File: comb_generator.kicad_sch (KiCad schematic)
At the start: 61 parts, among them J11 RFShield_TwoPieces, J2 RFShield_TwoPieces, U1 ISL3280ExHZ, U13 PAT1220-C-3DB, U2 PHA-13HLN+, U5 Si5351C-B-GM, U6 PHA-13HLN+, U7 PAT1220-C-3DB, Y2 TG2520SMN-xx.xxxxxxMhz-xxxxNM

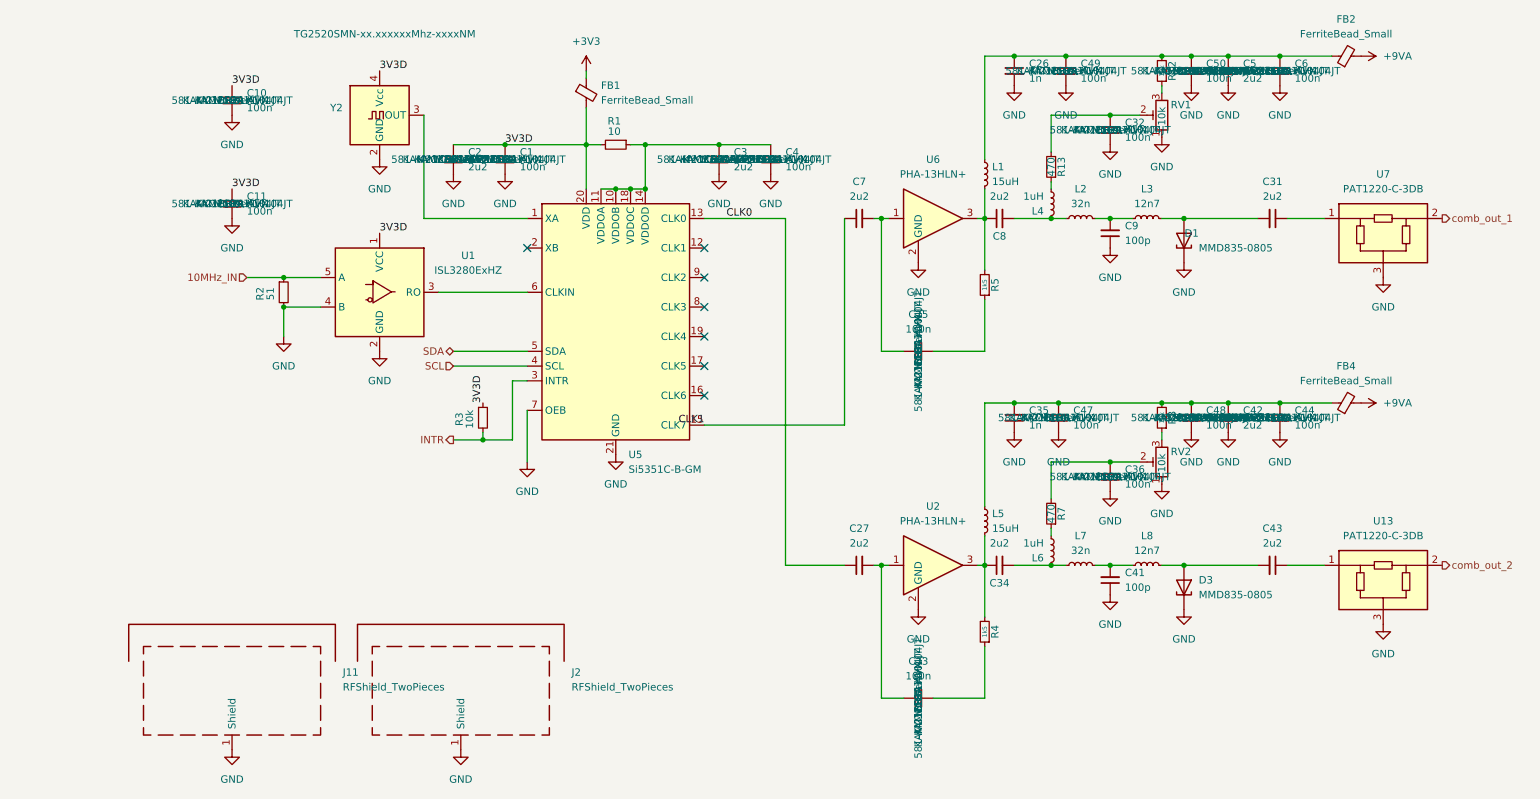
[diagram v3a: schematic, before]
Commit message: BOM...
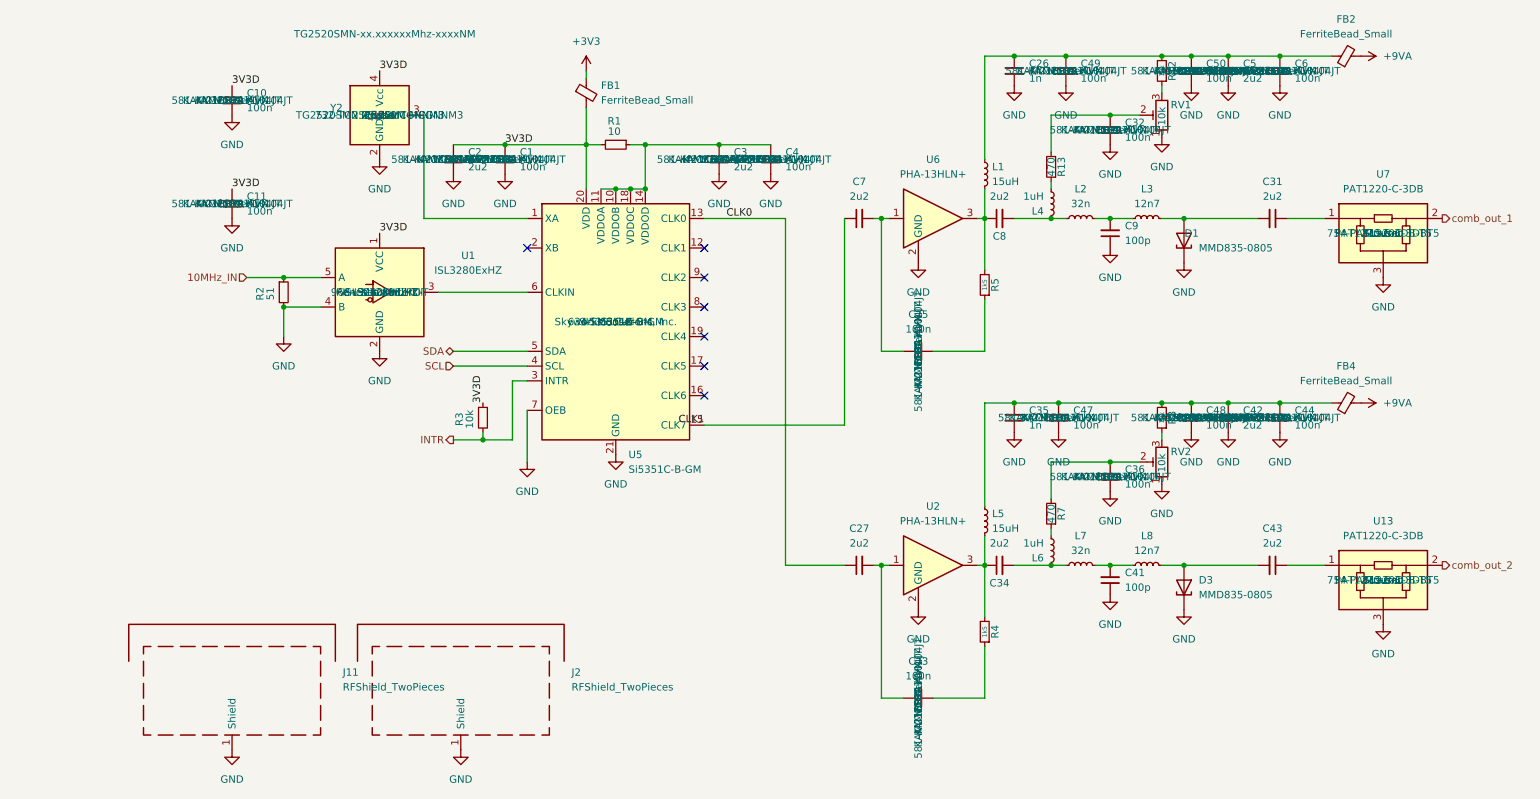
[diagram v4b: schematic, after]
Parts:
- RV1, RV2: Distributor (none) -> Mouser; Distributor PN (none) -> 652-TC33X-2-103E; Manufacturer (none) -> Bourns; Manufacturer PN (none) -> TC33X-2-103E
- U1: Distributor (none) -> Mouser; Distributor PN (none) -> 968-ISL3280EIHZ-T; Manufacturer (none) -> Renesas / Intersil; Manufacturer PN (none) -> ISL3280EIHZ-T
- U13, U7: Distributor (none) -> Mouser; Distributor PN (none) -> 754-PAT1220C-3DBT5; Manufacturer (none) -> Susumu; Manufacturer PN (none) -> PAT1220-C-3DB-T5
- U2, U6: Manufacturer (none) -> Mini-Circuits
- U5: Distributor (none) -> Mouser; Distributor PN (none) -> 634-SI5351C-B-GM; Manufacturer (none) -> Skyworks Solutions, Inc.; Manufacturer PN (none) -> SI5351C-B-GM
- Y2: Distributor (none) -> Mouser; Distributor PN (none) -> 732-TG252S25MCGNNM3; Manufacturer (none) -> Epson; Manufacturer PN (none) -> TG2520SMN 25.000M-MCGNNM3
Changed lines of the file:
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@@
 			)
 		)
+		(property "Distributor" "Mouser"
+			(at 74.93 88.9 0)
+			(effects
+				(font
+					(size 1.27 1.27)
+				)
+			)
+		)
+		(property "Distributor PN" "968-ISL3280EIHZ-T "
+			(at 74.93 88.9 0)
+			(effects
+				(font
+					(size 1.27 1.27)
+				)
+			)
+		)
+		(property "Manufacturer" "Renesas / Intersil "
+			(at 74.93 88.9 0)
+			(effects
+				(font
+					(size 1.27 1.27)
+				)
+			)
+		)
+		(property "Manufacturer PN" "ISL3280EIHZ-T "
+			(at 74.93 88.9 0)
+			(effects
+				(font
+					(size 1.27 1.27)
+				)
+			)
+		)
 		(pin "5"
 		)
@@
 			)
 		)
+		(property "Distributor" "Mouser"
+			(at 74.93 58.42 0)
+			(effects
+				(font
+					(size 1.27 1.27)
+				)
+			)
+		)
+		(property "Distributor PN" " 732-TG252S25MCGNNM3 "
+			(at 74.93 58.42 0)
+			(effects
+				(font
+					(size 1.27 1.27)
+				)
+			)
+		)
+		(property "Manufacturer" "Epson"
+			(at 74.93 58.42 0)
+			(effects
+				(font
+					(size 1.27 1.27)
+				)
+			)
+		)
+		(property "Manufacturer PN" "TG2520SMN 25.000M-MCGNNM3"
+			(at 74.93 58.42 0)
+			(effects
+				(font
+					(size 1.27 1.27)
+				)
+			)
+		)
 		(pin "2"
 		)
@@
 			)
 		)
+		(property "Distributor" "Mouser"
+			(at 115.57 93.98 0)
+			(effects
+				(font
+					(size 1.27 1.27)
+				)
+			)
+		)
+		(property "Distributor PN" " 634-SI5351C-B-GM "
+			(at 115.57 93.98 0)
+			(effects
+				(font
+					(size 1.27 1.27)
+				)
+			)
+		)
+		(property "Manufacturer" "Skyworks Solutions, Inc. "
+			(at 115.57 93.98 0)
+			(effects
+				(font
+					(size 1.27 1.27)
+				)
+			)
+		)
+		(property "Manufacturer PN" "SI5351C-B-GM"
+			(at 115.57 93.98 0)
+			(effects
+				(font
+					(size 1.27 1.27)
+				)
+			)
+		)
 		(pin "9"
 		)
@@
 			)
 		)
-		(property "Manufacturer PN" ""
+		(property "Manufacturer PN" "TC33X-2-103E"
 			(at 209.55 118.11 0)
 			(effects
@@
 			)
 		)
-		(property "Manufacturer" ""
+		(property "Manufacturer" "Bourns "
 			(at 209.55 118.11 0)
 			(effects
@@
 			)
 		)
-		(property "Distributor" ""
+		(property "Distributor" "Mouser"
 			(at 209.55 118.11 0)
 			(effects
@@
 			)
 		)
-		(property "Distributor PN" ""
+		(property "Distributor PN" " 652-TC33X-2-103E "
 			(at 209.55 118.11 0)
 			(effects
@@
 			)
 		)
-		(property "Manufacturer" ""
+		(property "Manufacturer" "Mini-Circuits"
 			(at 170.18 76.2 0)
 			(effects
@@
 			)
 		)
+		(property "Distributor" "Mouser"
+			(at 247.65 138.43 0)
+			(effects
+				(font
+					(size 1.27 1.27)
+				)
+			)
+		)
+		(property "Distributor PN" " 754-PAT1220C-3DBT5 "
+			(at 247.65 138.43 0)
+			(effects
+				(font
+					(size 1.27 1.27)
+				)
+			)
+		)
+		(property "Manufacturer" "Susumu "
+			(at 247.65 138.43 0)
+			(effects
+				(font
+					(size 1.27 1.27)
+				)
+			)
+		)
+		(property "Manufacturer PN" "PAT1220-C-3DB-T5"
+			(at 247.65 138.43 0)
+			(effects
+				(font
+					(size 1.27 1.27)
+				)
+			)
+		)
 		(pin "1"
 		)
@@
 			)
 		)
-		(property "Manufacturer PN" ""
+		(property "Manufacturer PN" "TC33X-2-103E"
 			(at 209.55 58.42 0)
 			(effects
@@
 			)
 		)
-		(property "Manufacturer" ""
+		(property "Manufacturer" "Bourns "
 			(at 209.55 58.42 0)
 			(effects
@@
 			)
 		)
-		(property "Distributor" ""
+		(property "Distributor" "Mouser"
 			(at 209.55 58.42 0)
 			(effects
@@
 			)
 		)
-		(property "Distributor PN" ""
+		(property "Distributor PN" " 652-TC33X-2-103E "
 			(at 209.55 58.42 0)
 			(effects
@@
 			)
 		)
-		(property "Manufacturer" ""
+		(property "Manufacturer" "Mini-Circuits"
 			(at 170.18 135.89 0)
 			(effects
@@
 			)
 		)
+		(property "Distributor" "Mouser"
+			(at 247.65 78.74 0)
+			(effects
+				(font
+					(size 1.27 1.27)
+				)
+			)
+		)
+		(property "Distributor PN" " 754-PAT1220C-3DBT5 "
+			(at 247.65 78.74 0)
+			(effects
+				(font
+					(size 1.27 1.27)
+				)
+			)
+		)
+		(property "Manufacturer" "Susumu "
+			(at 247.65 78.74 0)
+			(effects
+				(font
+					(size 1.27 1.27)
+				)
+			)
+		)
+		(property "Manufacturer PN" "PAT1220-C-3DB-T5"
+			(at 247.65 78.74 0)
+			(effects
+				(font
+					(size 1.27 1.27)
+				)
+			)
+		)
